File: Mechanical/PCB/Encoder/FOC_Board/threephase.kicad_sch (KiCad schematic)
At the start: 34 parts, among them Q1 CSD88537ND, Q2 CSD88537ND, Q3 CSD88537ND, U1 DRV8353RSRGZT

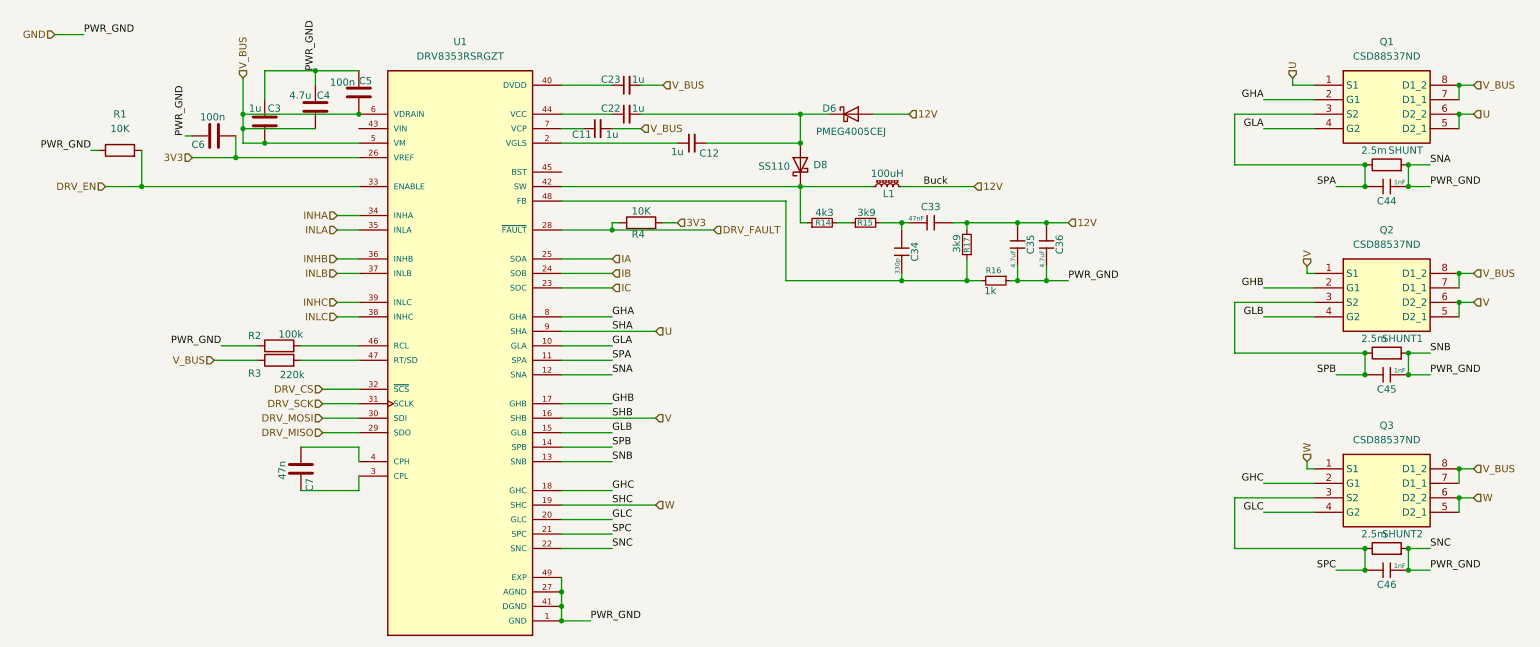
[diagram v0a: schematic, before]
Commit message: fix schematic
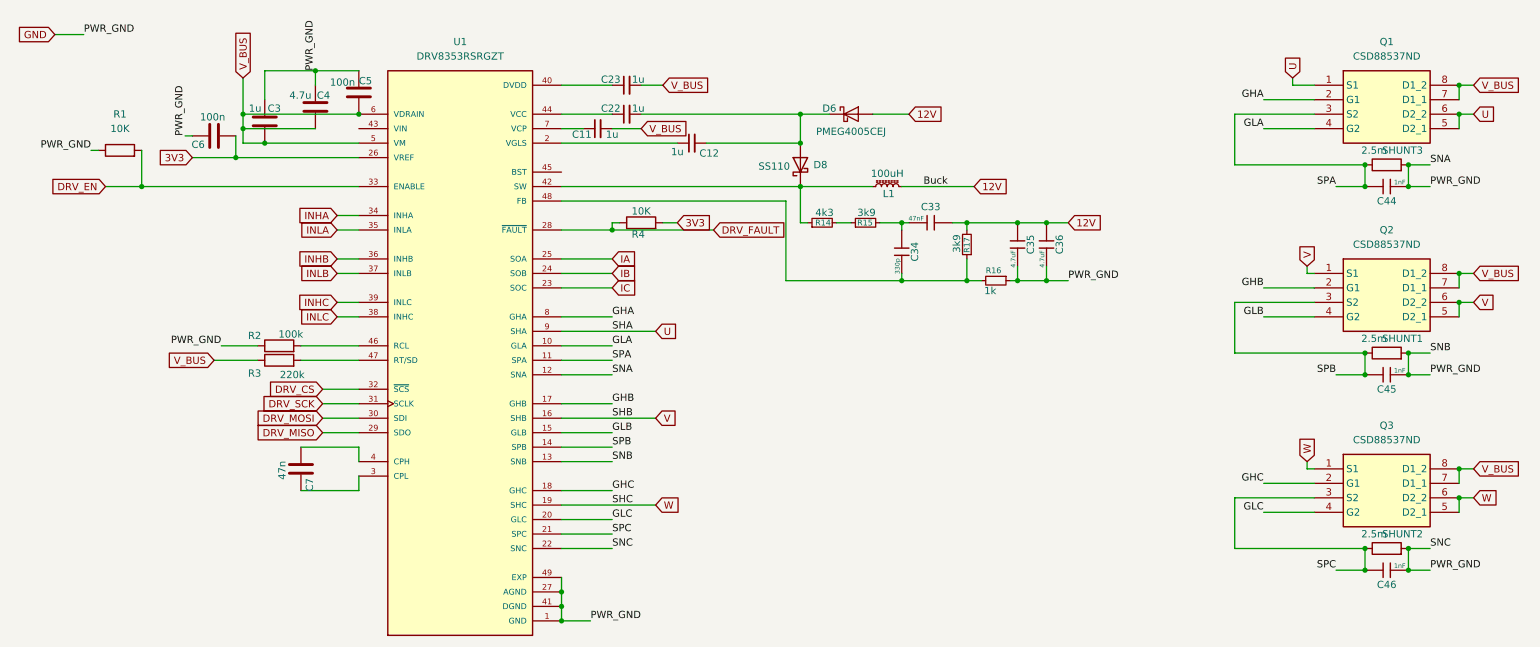
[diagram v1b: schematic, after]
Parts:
- Q1, Q2, Q3: footprint SOIC127P600X175-8N -> CSD88537ND:SOIC127P600X175-8N
- renumbered SHUNT to SHUNT3
